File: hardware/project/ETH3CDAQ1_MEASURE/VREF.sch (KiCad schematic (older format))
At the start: 12 parts, among them U801 OPA2277, U802 ADR4550

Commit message: Meas. module schematic design.
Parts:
- removed C801, C802, C803: 100n, Capacitor_SMD:C_0603_1608Metric_Pad1.08x0.95mm_HandSolder, symbol Device:C
- removed C806: 10u, Capacitor_SMD:C_1206_3216Metric_Pad1.33x1.80mm_HandSolder, symbol Device:C
- removed R802, R804: 10k, Resistor_SMD:R_0603_1608Metric_Pad0.98x0.95mm_HandSolder, symbol Device:R
- removed R803: 20k, Resistor_SMD:R_0603_1608Metric_Pad0.98x0.95mm_HandSolder, symbol Device:R
- removed U801: OPA2277, Package_SO:SOIC-8_3.9x4.9mm_P1.27mm, symbol Amplifier_Operational:OPA2277
- removed U802: ADR4550, Package_SO:SOIC-8_3.9x4.9mm_P1.27mm, symbol Reference_Voltage:ADR4550
- added C?: 1u, symbol Device:C
- added U802: REF5040ID, Package_SO:SOIC-8_3.9x4.9mm_P1.27mm, symbol Reference_Voltage:REF5040ID
- C804: value 10u -> 1u; footprint Capacitor_SMD:C_1206_3216Metric_Pad1.33x1.80mm_HandSolder -> (none)
- C805: value 100n -> 10u; footprint Capacitor_SMD:C_0603_1608Metric_Pad1.08x0.95mm_HandSolder -> (none)
- R801: value 10k -> 0R22; footprint Resistor_SMD:R_0603_1608Metric_Pad0.98x0.95mm_HandSolder -> (none)
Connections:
- net labels added: +5VF, VREF
- net labels removed: +10V, +15V, +5VP, +7.5V, -10V, -15V
- wire segments 46 -> 7
- no-connect marks 0 -> 1

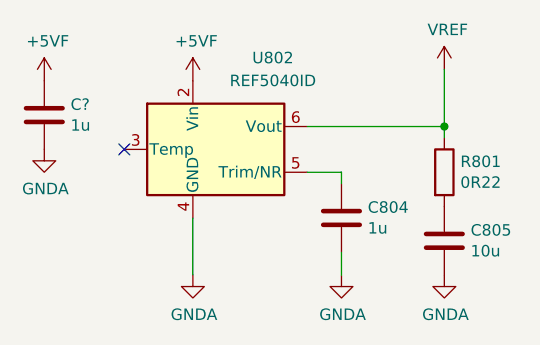
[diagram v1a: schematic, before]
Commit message: Measurement module development.
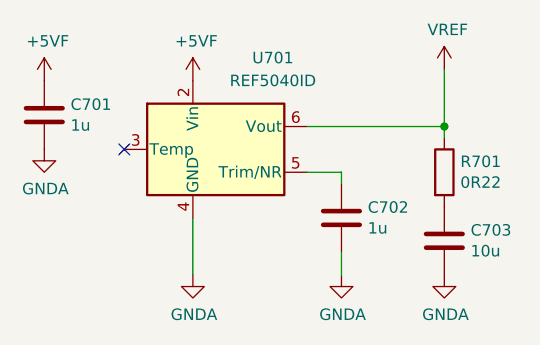
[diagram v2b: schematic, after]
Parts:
- C701: renamed from C?; footprint (none) -> Capacitor_SMD:C_0603_1608Metric_Pad1.08x0.95mm_HandSolder
- C702: renamed from C804; footprint (none) -> Capacitor_SMD:C_0603_1608Metric_Pad1.08x0.95mm_HandSolder
- C703: renamed from C805; footprint (none) -> Capacitor_SMD:C_0805_2012Metric_Pad1.18x1.45mm_HandSolder
- R701: renamed from R801; footprint (none) -> Resistor_SMD:R_0603_1608Metric_Pad0.98x0.95mm_HandSolder
- renumbered U802 to U701
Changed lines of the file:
@@
 $Descr A4 11693 8268
 encoding utf-8
-Sheet 8 10
+Sheet 7 15
 Title ""
 Date ""
@@
 $EndDescr
 $Comp
-L Reference_Voltage:REF5040ID U802
+L Reference_Voltage:REF5040ID U701
 U 1 1 5FEB8C44
 P 5750 3400
-F 0 "U802" H 6000 3800 50  0000 C CNN
+F 0 "U701" H 6000 3800 50  0000 C CNN
 F 1 "REF5040ID" H 6000 3700 50  0000 C CNN
 F 2 "Package_SO:SOIC-8_3.9x4.9mm_P1.27mm" H 5675 3150 50  0001 L CIN
@@
 $EndComp
 $Comp
-L power:GNDA #PWR0804
+L power:GNDA #PWR0704
 U 1 1 5FEB9127
 P 5650 3950
-F 0 "#PWR0804" H 5650 3700 50  0001 C CNN
+F 0 "#PWR0704" H 5650 3700 50  0001 C CNN
 F 1 "GNDA" H 5655 3777 50  0000 C CNN
 F 2 "" H 5650 3950 50  0001 C CNN
@@
 $EndComp
 $Comp
-L Device:C C804
+L Device:C C702
 U 1 1 5FEB948B
 P 6300 3700
-F 0 "C804" H 6415 3746 50  0000 L CNN
+F 0 "C702" H 6415 3746 50  0000 L CNN
 F 1 "1u" H 6415 3655 50  0000 L CNN
-F 2 "" H 6338 3550 50  0001 C CNN
+F 2 "Capacitor_SMD:C_0603_1608Metric_Pad1.08x0.95mm_HandSolder" H 6338 3550 50  0001 C CNN
 F 3 "~" H 6300 3700 50  0001 C CNN
 	1    6300 3700
@@
 	6300 3500 6150 3500
 $Comp
-L Device:R R801
+L Device:R R701
 U 1 1 5FEBB0E1
 P 6750 3500
-F 0 "R801" H 6820 3546 50  0000 L CNN
+F 0 "R701" H 6820 3546 50  0000 L CNN
 F 1 "0R22" H 6820 3455 50  0000 L CNN
-F 2 "" V 6680 3500 50  0001 C CNN
+F 2 "Resistor_SMD:R_0603_1608Metric_Pad0.98x0.95mm_HandSolder" V 6680 3500 50  0001 C CNN
 F 3 "~" H 6750 3500 50  0001 C CNN
 	1    6750 3500
@@
 $EndComp
 $Comp
-L Device:C C805
+L Device:C C703
 U 1 1 5FEBB94A
 P 6750 3800
-F 0 "C805" H 6865 3846 50  0000 L CNN
+F 0 "C703" H 6865 3846 50  0000 L CNN
 F 1 "10u" H 6865 3755 50  0000 L CNN
-F 2 "" H 6788 3650 50  0001 C CNN
+F 2 "Capacitor_SMD:C_0805_2012Metric_Pad1.18x1.45mm_HandSolder" H 6788 3650 50  0001 C CNN
 F 3 "~" H 6750 3800 50  0001 C CNN
 	1    6750 3800
@@
 	6750 3300 6150 3300
 $Comp
-L power:GNDA #PWR0807
+L power:GNDA #PWR0707
 U 1 1 5FEBCC1B
 P 6750 3950
-F 0 "#PWR0807" H 6750 3700 50  0001 C CNN
+F 0 "#PWR0707" H 6750 3700 50  0001 C CNN
 F 1 "GNDA" H 6755 3777 50  0000 C CNN
 F 2 "" H 6750 3950 50  0001 C CNN
@@
 	5650 3700 5650 3950
 $Comp
-L power:GNDA #PWR0805
+L power:GNDA #PWR0705
 U 1 1 5FEBCFC9
 P 6300 3950
-F 0 "#PWR0805" H 6300 3700 50  0001 C CNN
+F 0 "#PWR0705" H 6300 3700 50  0001 C CNN
 F 1 "GNDA" H 6305 3777 50  0000 C CNN
 F 2 "" H 6300 3950 50  0001 C CNN
@@
 NoConn ~ 5350 3400
 $Comp
-L ETH3CDAQ1:VREF #PWR0806
+L ETH3CDAQ1:VREF #PWR0706
 U 1 1 5FECCE94
 P 6750 3050
-F 0 "#PWR0806" H 6750 2900 50  0001 C CNN
+F 0 "#PWR0706" H 6750 2900 50  0001 C CNN
 F 1 "VREF" H 6765 3223 50  0000 C CNN
 F 2 "" H 6750 3050 50  0001 C CNN
@@
 P 5650 3100
 AR Path="/5FED0BD8/5FEE0464" Ref="#PWR?"  Part="1"
-AR Path="/5FC8249B/5FEE0464" Ref="#PWR0803"  Part="1"
-F 0 "#PWR0803" H 5650 2950 50  0001 C CNN
+AR Path="/5FC8249B/5FEE0464" Ref="#PWR0703"  Part="1"
+F 0 "#PWR0703" H 5650 2950 50  0001 C CNN
 F 1 "+5VF" H 5665 3273 50  0000 C CNN
 F 2 "" H 5650 3100 50  0001 C CNN
@@
 P 5000 3100
 AR Path="/5FED0BD8/5FFEBA4F" Ref="#PWR?"  Part="1"
-AR Path="/5FC8249B/5FFEBA4F" Ref="#PWR?"  Part="1"
-F 0 "#PWR?" H 5000 2950 50  0001 C CNN
+AR Path="/5FC8249B/5FFEBA4F" Ref="#PWR0701"  Part="1"
+F 0 "#PWR0701" H 5000 2950 50  0001 C CNN
 F 1 "+5VF" H 5015 3273 50  0000 C CNN
 F 2 "" H 5000 3100 50  0001 C CNN
@@
 $EndComp
 $Comp
-L Device:C C?
+L Device:C C701
 U 1 1 5FFEC0E9
 P 5000 3250
-F 0 "C?" H 5115 3296 50  0000 L CNN
+F 0 "C701" H 5115 3296 50  0000 L CNN
 F 1 "1u" H 5115 3205 50  0000 L CNN
-F 2 "" H 5038 3100 50  0001 C CNN
+F 2 "Capacitor_SMD:C_0603_1608Metric_Pad1.08x0.95mm_HandSolder" H 5038 3100 50  0001 C CNN
 F 3 "~" H 5000 3250 50  0001 C CNN
 	1    5000 3250
@@
 $EndComp
 $Comp
-L power:GNDA #PWR?
+L power:GNDA #PWR0702
 U 1 1 5FFEC27E
 P 5000 3400
-F 0 "#PWR?" H 5000 3150 50  0001 C CNN
+F 0 "#PWR0702" H 5000 3150 50  0001 C CNN
 F 1 "GNDA" H 5005 3227 50  0000 C CNN
 F 2 "" H 5000 3400 50  0001 C CNN

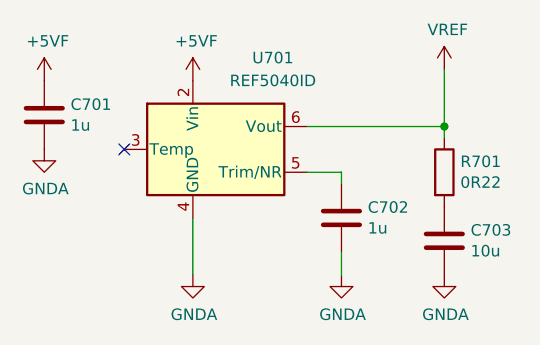
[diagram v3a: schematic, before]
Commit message: PCB layout
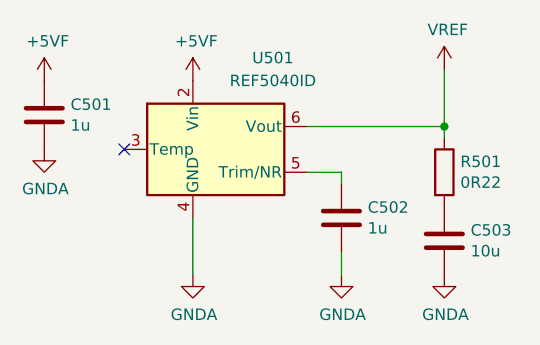
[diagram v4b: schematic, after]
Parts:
- renumbered C701 to C501, C702 to C502, C703 to C503, R701 to R501, U701 to U501
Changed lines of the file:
@@
 $EndDescr
 $Comp
-L Reference_Voltage:REF5040ID U701
+L Reference_Voltage:REF5040ID U501
 U 1 1 5FEB8C44
 P 5750 3400
-F 0 "U701" H 6000 3800 50  0000 C CNN
+F 0 "U501" H 6000 3800 50  0000 C CNN
 F 1 "REF5040ID" H 6000 3700 50  0000 C CNN
 F 2 "Package_SO:SOIC-8_3.9x4.9mm_P1.27mm" H 5675 3150 50  0001 L CIN
@@
 $EndComp
 $Comp
-L power:GNDA #PWR0704
+L power:GNDA #PWR0504
 U 1 1 5FEB9127
 P 5650 3950
-F 0 "#PWR0704" H 5650 3700 50  0001 C CNN
+F 0 "#PWR0504" H 5650 3700 50  0001 C CNN
 F 1 "GNDA" H 5655 3777 50  0000 C CNN
 F 2 "" H 5650 3950 50  0001 C CNN
@@
 $EndComp
 $Comp
-L Device:C C702
+L Device:C C502
 U 1 1 5FEB948B
 P 6300 3700
-F 0 "C702" H 6415 3746 50  0000 L CNN
+F 0 "C502" H 6415 3746 50  0000 L CNN
 F 1 "1u" H 6415 3655 50  0000 L CNN
 F 2 "Capacitor_SMD:C_0603_1608Metric_Pad1.08x0.95mm_HandSolder" H 6338 3550 50  0001 C CNN
@@
 	6300 3500 6150 3500
 $Comp
-L Device:R R701
+L Device:R R501
 U 1 1 5FEBB0E1
 P 6750 3500
-F 0 "R701" H 6820 3546 50  0000 L CNN
+F 0 "R501" H 6820 3546 50  0000 L CNN
 F 1 "0R22" H 6820 3455 50  0000 L CNN
 F 2 "Resistor_SMD:R_0603_1608Metric_Pad0.98x0.95mm_HandSolder" V 6680 3500 50  0001 C CNN
@@
 $EndComp
 $Comp
-L Device:C C703
+L Device:C C503
 U 1 1 5FEBB94A
 P 6750 3800
-F 0 "C703" H 6865 3846 50  0000 L CNN
+F 0 "C503" H 6865 3846 50  0000 L CNN
 F 1 "10u" H 6865 3755 50  0000 L CNN
 F 2 "Capacitor_SMD:C_0805_2012Metric_Pad1.18x1.45mm_HandSolder" H 6788 3650 50  0001 C CNN
@@
 	6750 3300 6150 3300
 $Comp
-L power:GNDA #PWR0707
+L power:GNDA #PWR0507
 U 1 1 5FEBCC1B
 P 6750 3950
-F 0 "#PWR0707" H 6750 3700 50  0001 C CNN
+F 0 "#PWR0507" H 6750 3700 50  0001 C CNN
 F 1 "GNDA" H 6755 3777 50  0000 C CNN
 F 2 "" H 6750 3950 50  0001 C CNN
@@
 	5650 3700 5650 3950
 $Comp
-L power:GNDA #PWR0705
+L power:GNDA #PWR0505
 U 1 1 5FEBCFC9
 P 6300 3950
-F 0 "#PWR0705" H 6300 3700 50  0001 C CNN
+F 0 "#PWR0505" H 6300 3700 50  0001 C CNN
 F 1 "GNDA" H 6305 3777 50  0000 C CNN
 F 2 "" H 6300 3950 50  0001 C CNN
@@
 NoConn ~ 5350 3400
 $Comp
-L ETH3CDAQ1:VREF #PWR0706
+L ETH3CDAQ1:VREF #PWR0506
 U 1 1 5FECCE94
 P 6750 3050
-F 0 "#PWR0706" H 6750 2900 50  0001 C CNN
+F 0 "#PWR0506" H 6750 2900 50  0001 C CNN
 F 1 "VREF" H 6765 3223 50  0000 C CNN
 F 2 "" H 6750 3050 50  0001 C CNN
@@
 P 5650 3100
 AR Path="/5FED0BD8/5FEE0464" Ref="#PWR?"  Part="1"
-AR Path="/5FC8249B/5FEE0464" Ref="#PWR0703"  Part="1"
-F 0 "#PWR0703" H 5650 2950 50  0001 C CNN
+AR Path="/5FC8249B/5FEE0464" Ref="#PWR0503"  Part="1"
+F 0 "#PWR0503" H 5650 2950 50  0001 C CNN
 F 1 "+5VF" H 5665 3273 50  0000 C CNN
 F 2 "" H 5650 3100 50  0001 C CNN
@@
 P 5000 3100
 AR Path="/5FED0BD8/5FFEBA4F" Ref="#PWR?"  Part="1"
-AR Path="/5FC8249B/5FFEBA4F" Ref="#PWR0701"  Part="1"
-F 0 "#PWR0701" H 5000 2950 50  0001 C CNN
+AR Path="/5FC8249B/5FFEBA4F" Ref="#PWR0501"  Part="1"
+F 0 "#PWR0501" H 5000 2950 50  0001 C CNN
 F 1 "+5VF" H 5015 3273 50  0000 C CNN
 F 2 "" H 5000 3100 50  0001 C CNN
@@
 $EndComp
 $Comp
-L Device:C C701
+L Device:C C501
 U 1 1 5FFEC0E9
 P 5000 3250
-F 0 "C701" H 5115 3296 50  0000 L CNN
+F 0 "C501" H 5115 3296 50  0000 L CNN
 F 1 "1u" H 5115 3205 50  0000 L CNN
 F 2 "Capacitor_SMD:C_0603_1608Metric_Pad1.08x0.95mm_HandSolder" H 5038 3100 50  0001 C CNN
@@
 $EndComp
 $Comp
-L power:GNDA #PWR0702
+L power:GNDA #PWR0502
 U 1 1 5FFEC27E
 P 5000 3400
-F 0 "#PWR0702" H 5000 3150 50  0001 C CNN
+F 0 "#PWR0502" H 5000 3150 50  0001 C CNN
 F 1 "GNDA" H 5005 3227 50  0000 C CNN
 F 2 "" H 5000 3400 50  0001 C CNN
